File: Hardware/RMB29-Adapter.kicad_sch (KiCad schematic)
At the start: 14 parts, among them J1 CONN IN, J2 CONN OUT, U1 MCP602, U2 MCP602

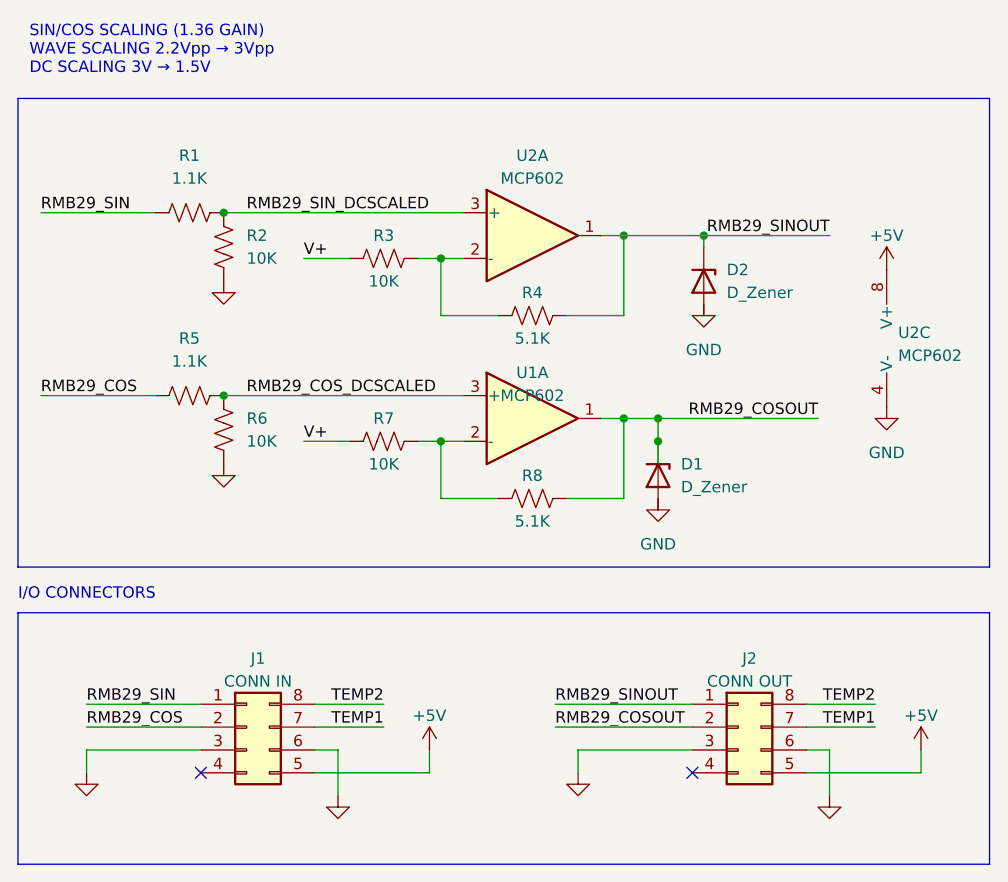
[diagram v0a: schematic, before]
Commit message: Missing connections
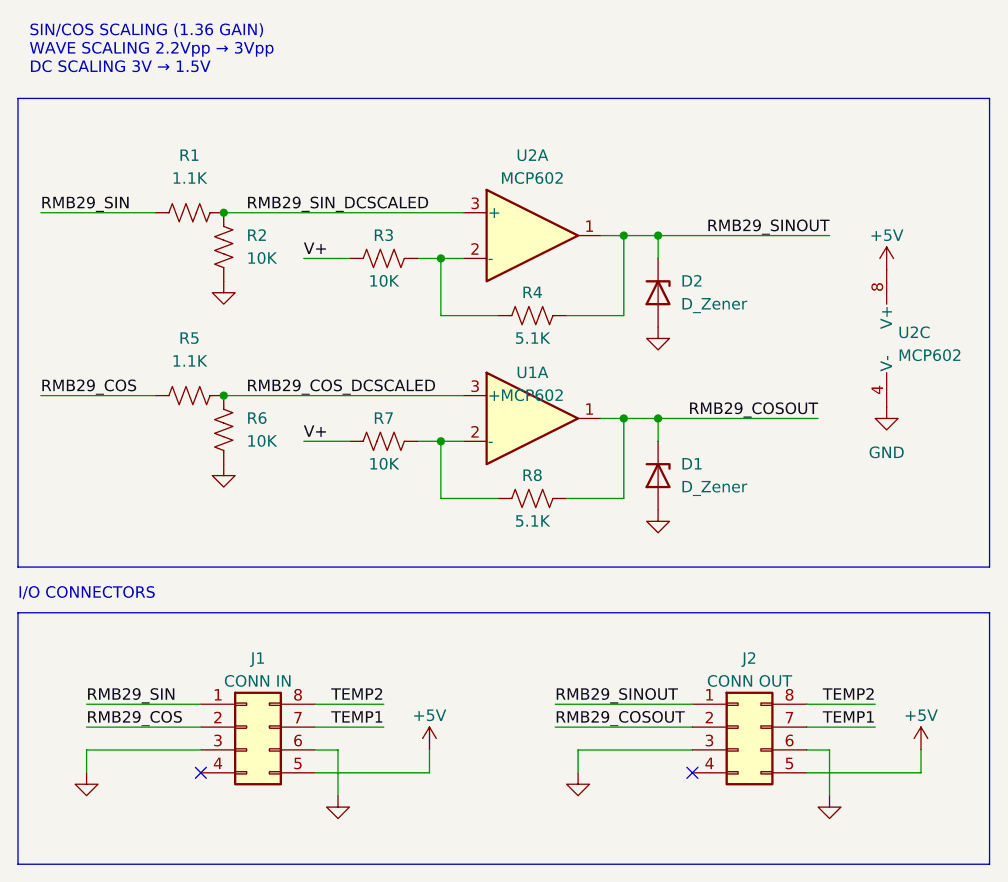
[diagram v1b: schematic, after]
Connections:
- net GND: now also D1.2 (A), D2.2 (A)
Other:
- moved on the sheet: D2
